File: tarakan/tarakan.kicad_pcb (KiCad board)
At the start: 2 copper layers, 48 x 48 mm, 30 parts, among them J1 power_in, J2 signal, J3 prog_header, J4 MOTOR1, J5 MOTOR2, U1 HT7550-1, U2 VNH7100AS, U3 ATtiny1617-M, U4 VNH7100AS

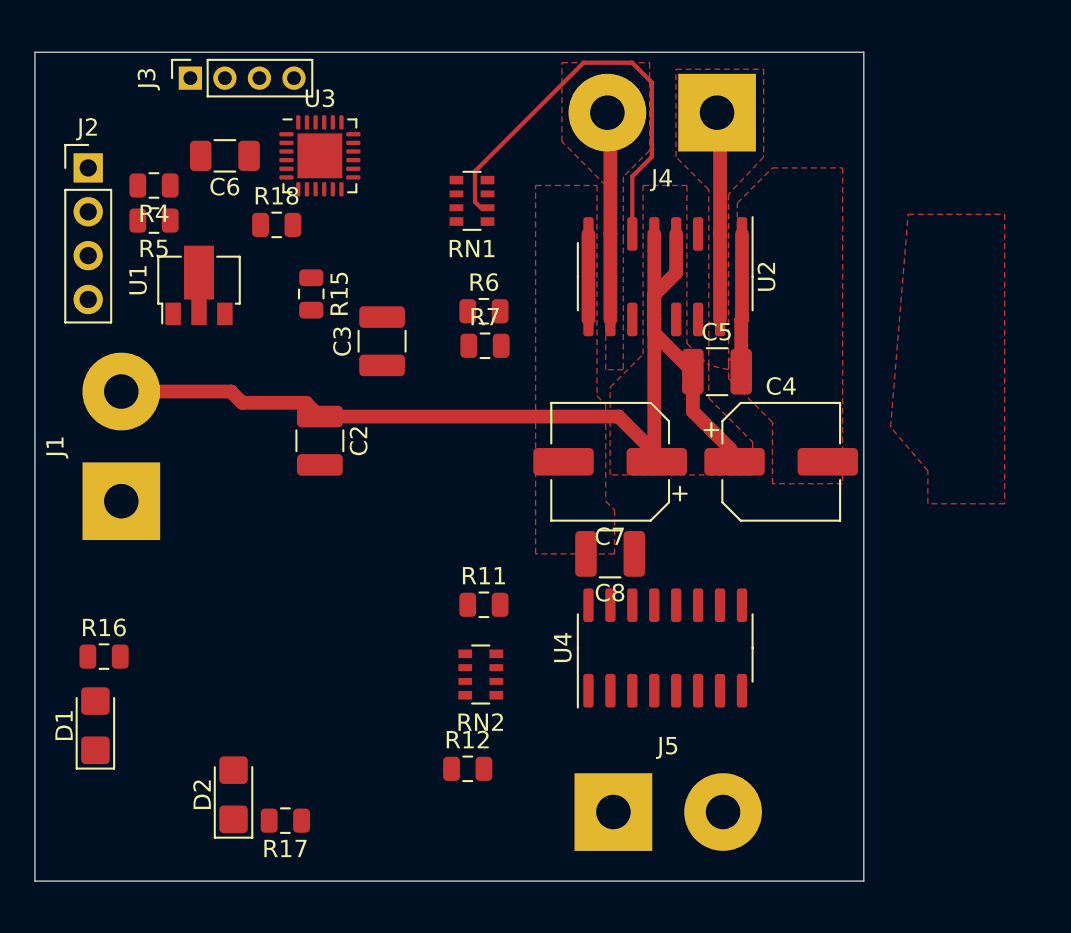
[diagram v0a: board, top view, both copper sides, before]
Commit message: is it a beetle esc?
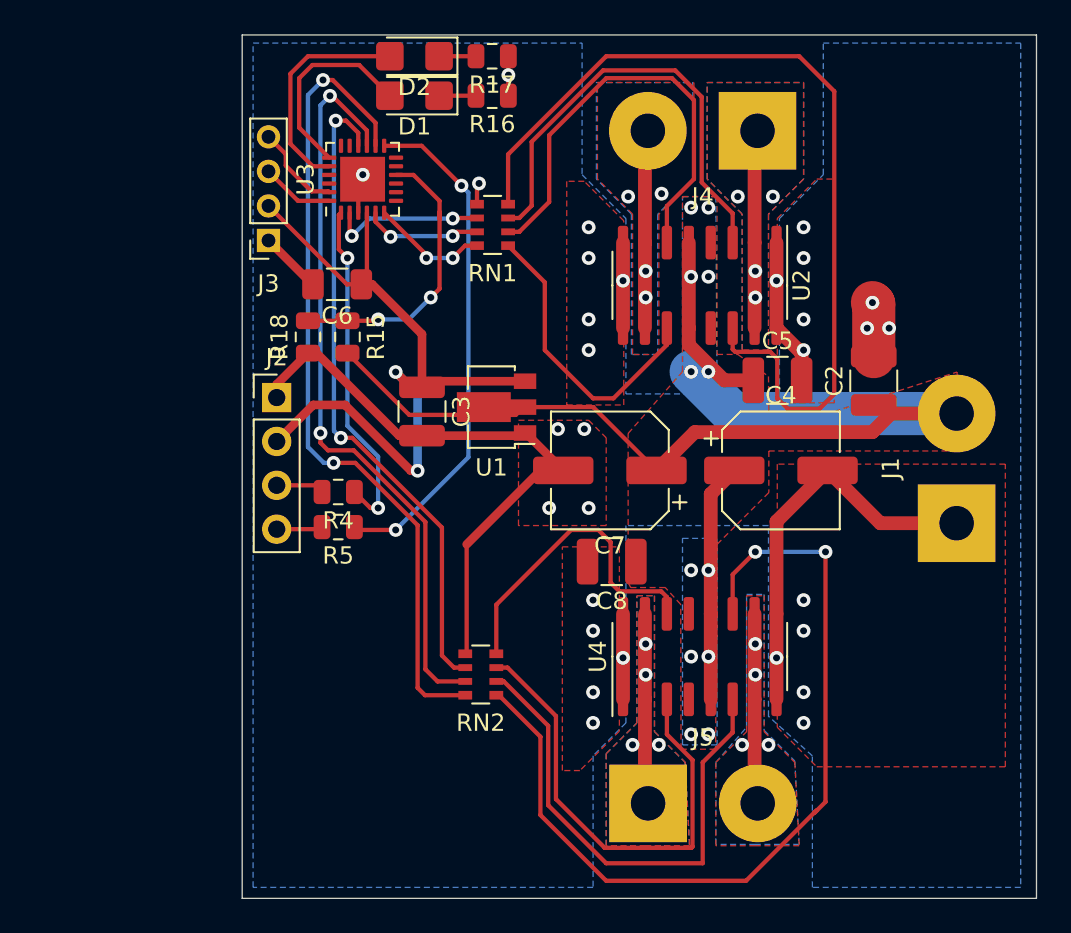
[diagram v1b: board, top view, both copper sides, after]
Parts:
- removed R11, R6: 10k, Resistor_SMD:R_0805_2012Metric
- removed R12, R7: 1k, Resistor_SMD:R_0805_2012Metric
- moved J1 48.4 mm to (150.9, 96.8)
- moved R17 45.9 mm to (124.0, 69.7)
- moved D2 44.0 mm to (119.5, 69.7), turned to 180 degrees
- moved D1 40.9 mm to (119.5, 72.0), turned to 180 degrees
- moved R16 39.5 mm to (124.0, 72.0), turned to 180 degrees
- moved C2 32.3 mm to (146.1, 88.5), turned to 90 degrees
- moved R4 20.7 mm to (115.1, 95.0)
- moved R5 20.7 mm to (115.1, 97.0)
- moved U1 18.6 mm to (124.2, 90.1), turned to 180 degrees
- moved J2 17.2 mm to (111.5, 89.5)
- moved J3 10.4 mm to (111.0, 80.4), turned to 180 degrees
- moved C6 9.88 mm to (115.0, 82.9)
- moved R18 6.74 mm to (113.3, 86.0), turned to 90 degrees
- moved C3 4.68 mm to (119.9, 90.3), turned to -90 degrees
- moved C5 3.54 mm to (140.5, 88.5)
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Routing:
- net GND: track 12.9 -> 88.9 mm, vias 0 -> 30
- net Net-(RN1-Pad4): track 0.00 -> 52.7 mm
- net Net-(RN2-Pad1): track 0.00 -> 50.9 mm, vias 0 -> 2
- net MOTOR2PWM: track 0.00 -> 47.6 mm, vias 0 -> 2
- net VLOGIC: track 0.00 -> 44.2 mm, vias 0 -> 2
- net MOTOR2B: track 0.00 -> 43.3 mm, vias 0 -> 2
- net MOTOR2A: track 0.00 -> 38.0 mm, vias 0 -> 2
- net Net-(R5-Pad1): track 0.00 -> 29.7 mm, vias 0 -> 2
- net Net-(RN2-Pad2): track 0.00 -> 29.2 mm
- net Net-(RN2-Pad3): track 0.00 -> 27.7 mm
- net Net-(RN1-Pad3): track 0.00 -> 26.7 mm
- net VBAT: track 59.5 -> 80.5 mm, vias 0 -> 12
- net Net-(R4-Pad1): track 0.00 -> 19.9 mm, vias 0 -> 2
- net Net-(RN2-Pad4): track 0.00 -> 18.5 mm
- net Net-(RN1-Pad1): track 0.00 -> 17.4 mm
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- added copper zone on B.Cu, net /M1OUTA
- added copper zone on B.Cu, net /M1OUTB
- added copper zone on B.Cu, net /M2OUTA
- added copper zone on F.Cu, net /M2OUTA
- added copper zone on B.Cu, net /M2OUTB
- added copper zone on F.Cu, net /M2OUTB
- added copper zone on B.Cu, net GND
- added copper zone on B.Cu, net VBAT
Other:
- board size 48 x 48 mm -> 46 x 50 mm
- board text added: "Add screw holes"
- board text added: "Move C2 to less stupid place Check terminal blocks fit power connectors"
- board text added: "move leds away from edge"
- board text added: "move power terminals in slightly; shrink board 1mm"
